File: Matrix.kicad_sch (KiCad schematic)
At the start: 106 parts, among them SW3 RotaryEncoder_Switch

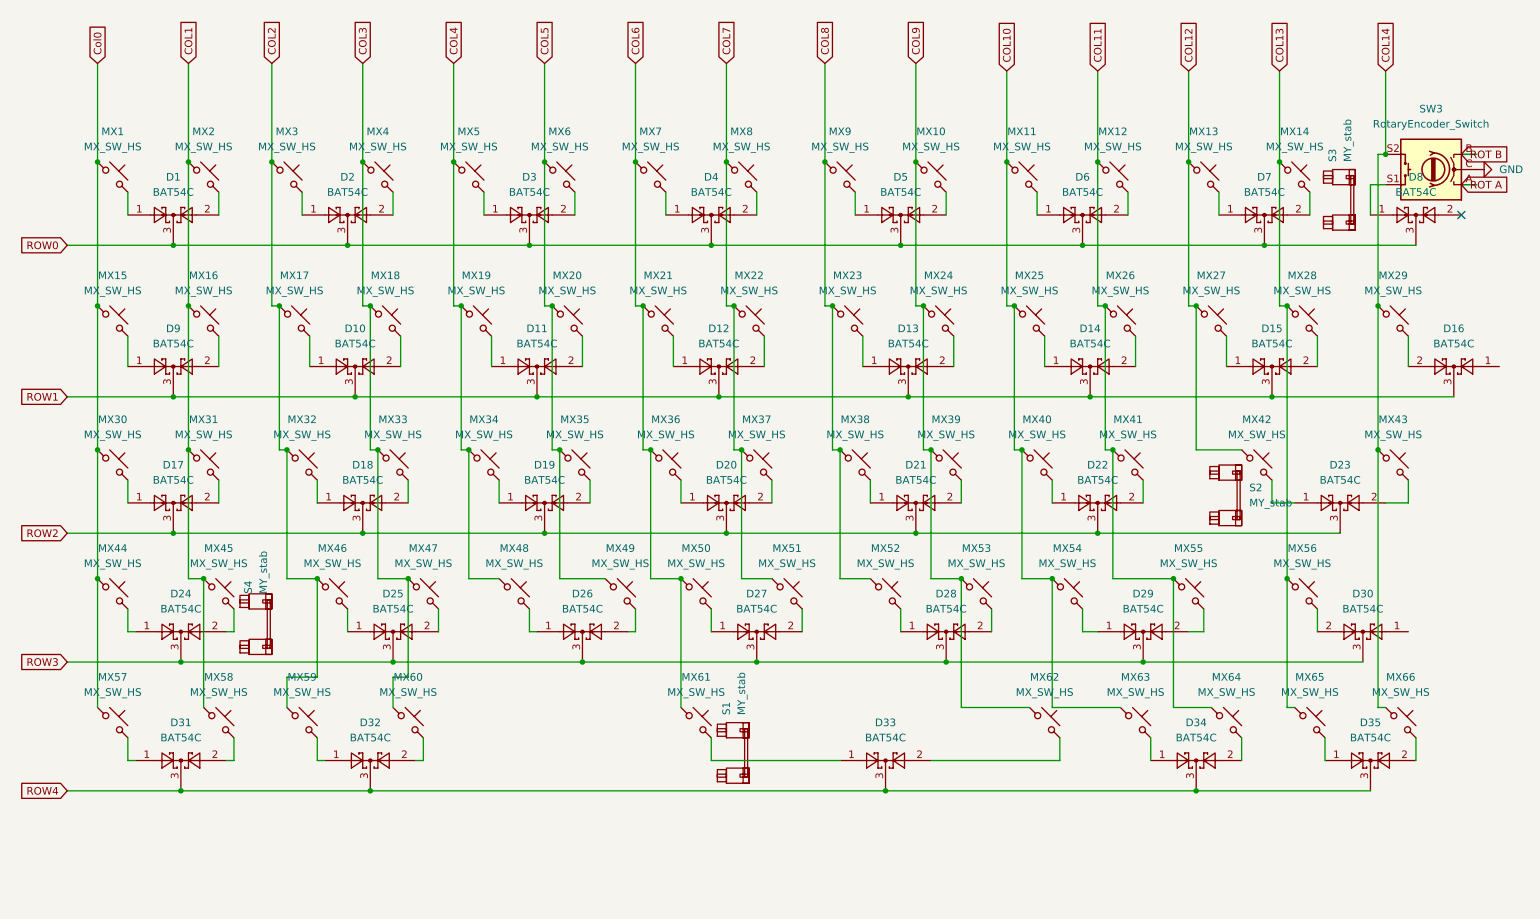
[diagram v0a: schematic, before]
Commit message: Routed more of matrix; Grounded
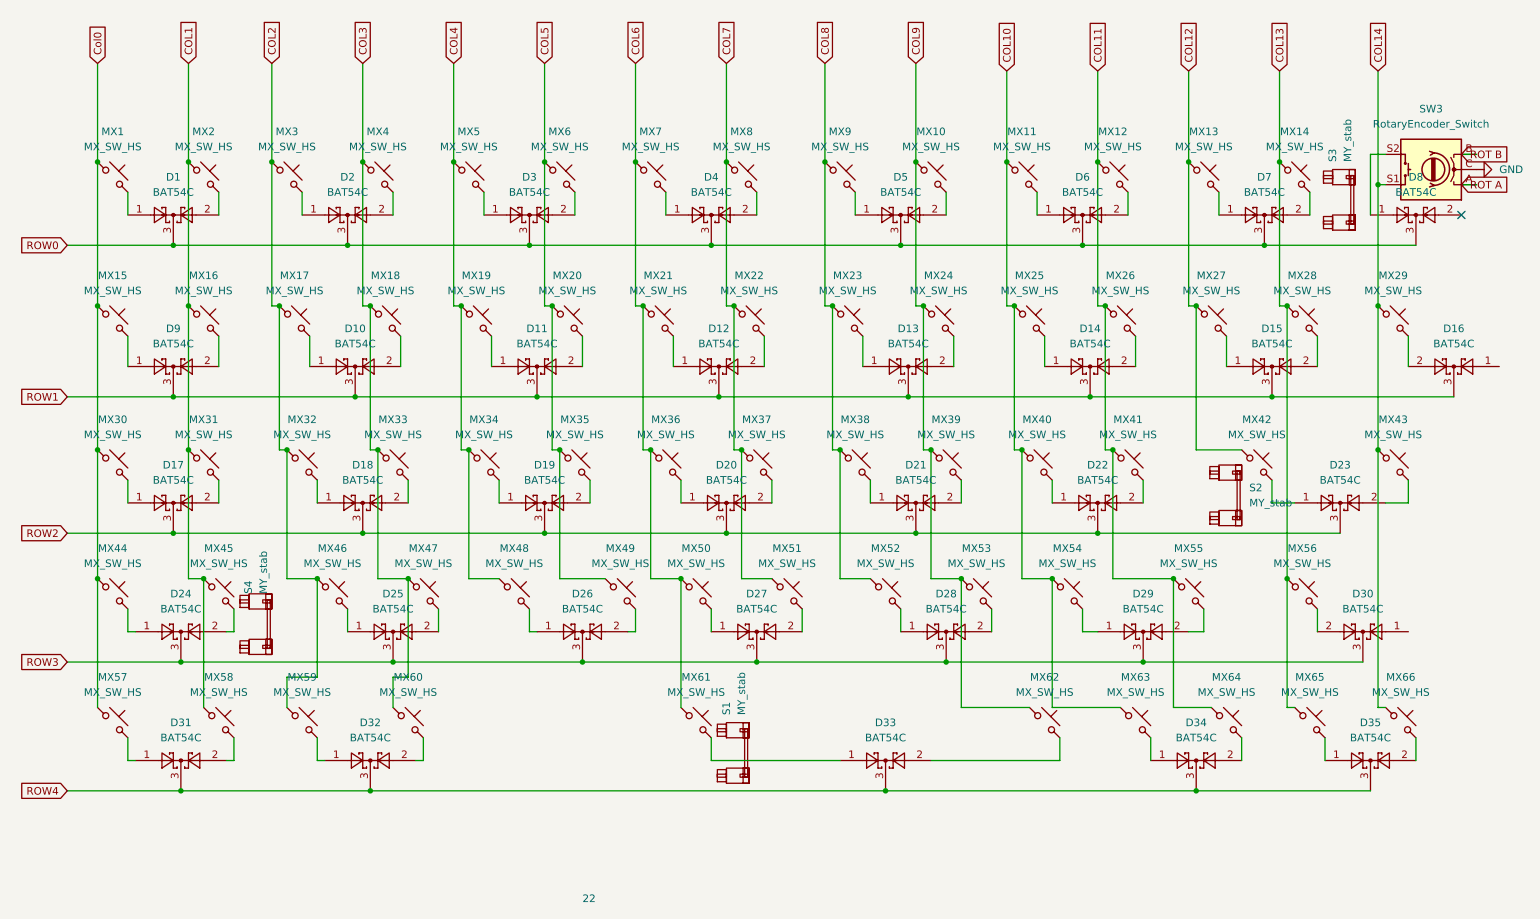
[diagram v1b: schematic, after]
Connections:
- net COL14: now also SW3.S1; no longer SW3.S2
- net at D8.1: now also SW3.S2; no longer SW3.S1
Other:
- note added: "22"
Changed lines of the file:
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@@
   (junction (at 99.06 63.5) (diameter 0) (color 0 0 0 0)
   )
+  (junction (at 241.3 53.34) (diameter 0) (color 0 0 0 0)
+  )
   (junction (at 69.85 88.9) (diameter 0) (color 0 0 0 0)
   )
@@
   )
   (junction (at 162.56 88.9) (diameter 0) (color 0 0 0 0)
-  )
-  (junction (at 242.57 48.26) (diameter 0) (color 0 0 0 0)
   )
   (junction (at 39.37 111.76) (diameter 0) (color 0 0 0 0)
@@
     (stroke (width 0) (type default))
   )
+  (wire (pts (xy 241.3 53.34) (xy 242.57 53.34))
+    (stroke (width 0) (type default))
+  )
   (wire (pts (xy 116.84 33.02) (xy 116.84 49.53))
     (stroke (width 0) (type default))
@@
     (stroke (width 0) (type default))
   )
-  (wire (pts (xy 241.3 48.26) (xy 241.3 73.66))
+  (wire (pts (xy 241.3 34.29) (xy 241.3 53.34))
     (stroke (width 0) (type default))
   )
@@
     (stroke (width 0) (type default))
   )
-  (wire (pts (xy 242.57 53.34) (xy 240.03 53.34))
+  (wire (pts (xy 242.57 48.26) (xy 240.03 48.26))
     (stroke (width 0) (type default))
   )
@@
     (stroke (width 0) (type default))
   )
-  (wire (pts (xy 241.3 48.26) (xy 242.57 48.26))
-    (stroke (width 0) (type default))
-  )
   (wire (pts (xy 151.13 119.38) (xy 156.21 119.38))
     (stroke (width 0) (type default))
@@
     (stroke (width 0) (type default))
   )
-  (wire (pts (xy 242.57 34.29) (xy 242.57 48.26))
-    (stroke (width 0) (type default))
-  )
   (wire (pts (xy 186.69 102.87) (xy 186.69 106.68))
     (stroke (width 0) (type default))
@@
     (stroke (width 0) (type default))
   )
-  (wire (pts (xy 240.03 53.34) (xy 240.03 58.42))
+  (wire (pts (xy 240.03 48.26) (xy 240.03 58.42))
     (stroke (width 0) (type default))
   )
@@
     (stroke (width 0) (type default))
   )
+  (wire (pts (xy 241.3 53.34) (xy 241.3 73.66))
+    (stroke (width 0) (type default))
+  )
   (wire (pts (xy 55.88 73.66) (xy 57.15 73.66))
     (stroke (width 0) (type default))
@@
   (wire (pts (xy 154.94 78.74) (xy 154.94 83.82))
     (stroke (width 0) (type default))
+  )
+  (text "22" (at 107.95 173.99 0)
+    (effects (font (size 1.27 1.27)) (justify left bottom))
   )
   (global_label "COL3" (shape input) (at 71.12 33.02 90) (fields_autoplaced)
@@
     )
   )
-  (global_label "COL14" (shape input) (at 242.57 34.29 90) (fields_autoplaced)
-    (effects (font (size 1.27 1.27)) (justify left))
-    (property "Intersheetrefs" "${INTERSHEET_REFS}" (at 242.57 25.2572 90)
-      (effects (font (size 1.27 1.27)) (justify left) hide)
-    )
+  (global_label "COL14" (shape input) (at 241.3 34.29 90) (fields_autoplaced)
+    (effects (font (size 1.27 1.27)) (justify left))
+    (property "Intersheetrefs" "${INTERSHEET_REFS}" (at 241.3 25.2572 90)
+      (effects (font (size 1.27 1.27)) (justify left) hide)
+    )
